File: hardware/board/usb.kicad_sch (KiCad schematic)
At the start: 30 parts, among them J3 USB3_A, U1 RK3568, U14 ESD5311X, U15 ESD5311X, U16 ESD5311X, U17 ESD5311X, U18 SY6280AAC

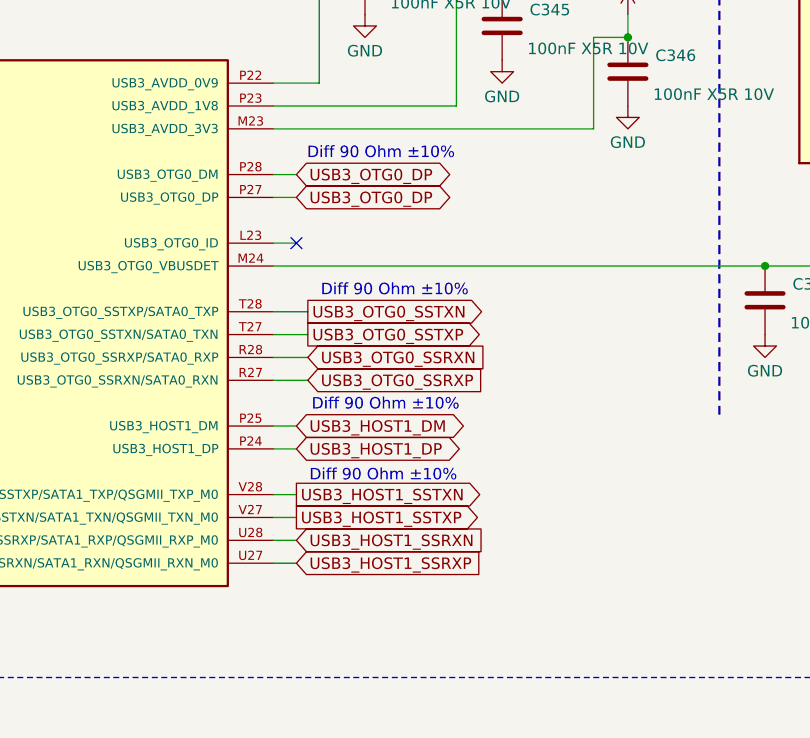
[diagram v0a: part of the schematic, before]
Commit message: did a thing
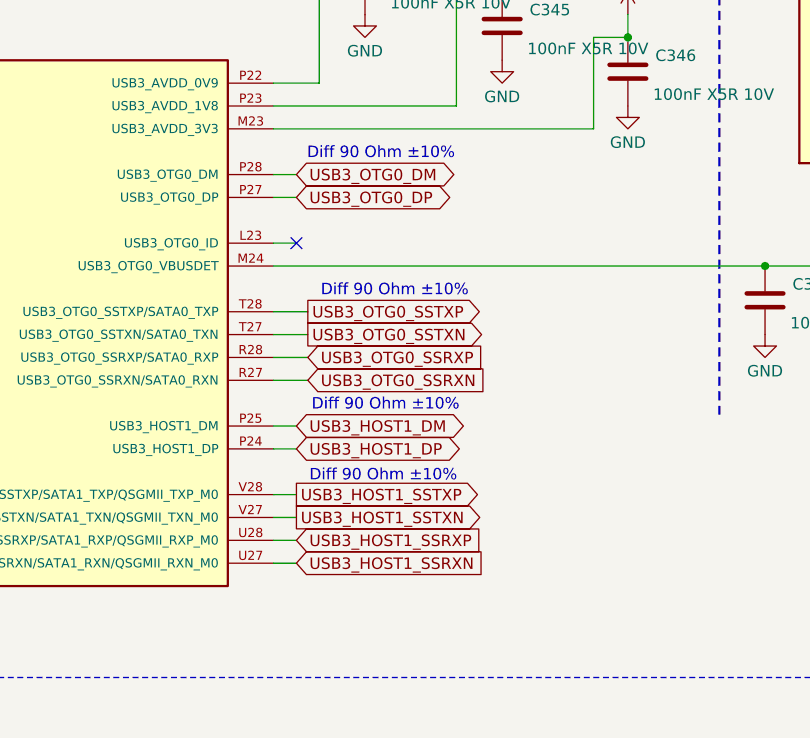
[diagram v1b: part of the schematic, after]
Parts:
- J3: footprint (none) -> lcsc:USB-A-SMD_U-A-39SS-W-1
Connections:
- net USB3_HOST1_SSRXN: now also U1.U27 (USB3_HOST1_SSRXN/SATA1_RXN/QSGMII_RXN_M0); no longer U1.U28 (USB3_HOST1_SSRXP/SATA1_RXP/QSGMII_RXP_M0)
- net USB3_HOST1_SSRXP: now also U1.U28 (USB3_HOST1_SSRXP/SATA1_RXP/QSGMII_RXP_M0); no longer U1.U27 (USB3_HOST1_SSRXN/SATA1_RXN/QSGMII_RXN_M0)
- net USB3_HOST1_SSTXN: now also U1.V27 (USB3_HOST1_SSTXN/SATA1_TXN/QSGMII_TXN_M0); no longer U1.V28 (USB3_HOST1_SSTXP/SATA1_TXP/QSGMII_TXP_M0)
- net USB3_HOST1_SSTXP: now also U1.V28 (USB3_HOST1_SSTXP/SATA1_TXP/QSGMII_TXP_M0); no longer U1.V27 (USB3_HOST1_SSTXN/SATA1_TXN/QSGMII_TXN_M0)
- net USB3_OTG0_DP: no longer U1.P28 (USB3_OTG0_DM)
- net USB3_OTG0_SSRXN: now also U1.R27 (USB3_OTG0_SSRXN/SATA0_RXN); no longer U1.R28 (USB3_OTG0_SSRXP/SATA0_RXP)
- net USB3_OTG0_SSRXP: now also U1.R28 (USB3_OTG0_SSRXP/SATA0_RXP); no longer U1.R27 (USB3_OTG0_SSRXN/SATA0_RXN)
- net USB3_OTG0_SSTXN: now also U1.T27 (USB3_OTG0_SSTXN/SATA0_TXN); no longer U1.T28 (USB3_OTG0_SSTXP/SATA0_TXP)
- net USB3_OTG0_SSTXP: now also U1.T28 (USB3_OTG0_SSTXP/SATA0_TXP); no longer U1.T27 (USB3_OTG0_SSTXN/SATA0_TXN)
- new net USB3_OTG0_DM: U1.P28 (USB3_OTG0_DM)
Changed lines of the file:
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@@
 	(global_label "USB3_HOST1_SSTXP"
 		(shape output)
-		(at 193.04 88.9 0)
+		(at 193.04 86.36 0)
 		(fields_autoplaced yes)
 		(effects
@@
 		)
 		(property "Intersheetrefs" "${INTERSHEET_REFS}"
-			(at 214.8936 88.9 0)
+			(at 214.8936 86.36 0)
 			(effects
 				(font
@@
 	(global_label "USB3_HOST1_SSRXN"
 		(shape input)
-		(at 193.04 91.44 0)
+		(at 193.04 93.98 0)
 		(fields_autoplaced yes)
 		(effects
@@
 		)
 		(property "Intersheetrefs" "${INTERSHEET_REFS}"
-			(at 215.2565 91.44 0)
+			(at 215.2565 93.98 0)
 			(effects
 				(font
@@
 	(global_label "USB3_HOST1_SSRXP"
 		(shape input)
-		(at 193.04 93.98 0)
+		(at 193.04 91.44 0)
 		(fields_autoplaced yes)
 		(effects
@@
 		)
 		(property "Intersheetrefs" "${INTERSHEET_REFS}"
-			(at 215.196 93.98 0)
+			(at 215.196 91.44 0)
 			(effects
 				(font
@@
 	(global_label "USB3_OTG0_SSTXP"
 		(shape output)
-		(at 194.31 68.58 0)
+		(at 194.31 66.04 0)
 		(fields_autoplaced yes)
 		(effects
@@
 		)
 		(property "Intersheetrefs" "${INTERSHEET_REFS}"
-			(at 214.8936 68.58 0)
+			(at 214.8936 66.04 0)
 			(effects
 				(font
@@
 	(global_label "USB3_OTG0_SSRXP"
 		(shape input)
-		(at 194.31 73.66 0)
+		(at 194.31 71.12 0)
 		(fields_autoplaced yes)
 		(effects
@@
 		)
 		(property "Intersheetrefs" "${INTERSHEET_REFS}"
-			(at 215.196 73.66 0)
+			(at 215.196 71.12 0)
 			(effects
 				(font
@@
 		)
 	)
-	(global_label "USB3_OTG0_DP"
+	(global_label "USB3_OTG0_DM"
 		(shape bidirectional)
 		(at 193.04 50.8 0)
@@
 		)
 		(property "Intersheetrefs" "${INTERSHEET_REFS}"
-			(at 211.4088 50.8 0)
+			(at 211.5902 50.8 0)
 			(effects
 				(font
@@
 	(global_label "USB3_OTG0_SSRXN"
 		(shape input)
-		(at 194.31 71.12 0)
+		(at 194.31 73.66 0)
 		(fields_autoplaced yes)
 		(effects
@@
 		)
 		(property "Intersheetrefs" "${INTERSHEET_REFS}"
-			(at 215.2565 71.12 0)
+			(at 215.2565 73.66 0)
 			(effects
 				(font
@@
 	(global_label "USB3_OTG0_SSTXN"
 		(shape output)
-		(at 194.31 66.04 0)
+		(at 194.31 68.58 0)
 		(fields_autoplaced yes)
 		(effects
@@
 		)
 		(property "Intersheetrefs" "${INTERSHEET_REFS}"
-			(at 214.9541 66.04 0)
+			(at 214.9541 68.58 0)
 			(effects
 				(font
@@
 	(global_label "USB3_HOST1_SSTXN"
 		(shape output)
-		(at 193.04 86.36 0)
+		(at 193.04 88.9 0)
 		(fields_autoplaced yes)
 		(effects
@@
 		)
 		(property "Intersheetrefs" "${INTERSHEET_REFS}"
-			(at 214.9541 86.36 0)
+			(at 214.9541 88.9 0)
 			(effects
 				(font
@@
 			)
 		)
-		(property "Footprint" ""
+		(property "Footprint" "lcsc:USB-A-SMD_U-A-39SS-W-1"
 			(at 44.45 157.48 0)
 			(effects
